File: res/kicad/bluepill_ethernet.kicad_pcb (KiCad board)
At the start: 2 copper layers, 50.4 x 48 mm, 23 parts, among them J1 HEADER-1x20, J2 Conn_01x03, J3 Conn_02x05_Odd_Even, SW1 SW_Push, U1 BluePill_STM32F103C, U2 93C46, U3 WIZ850io

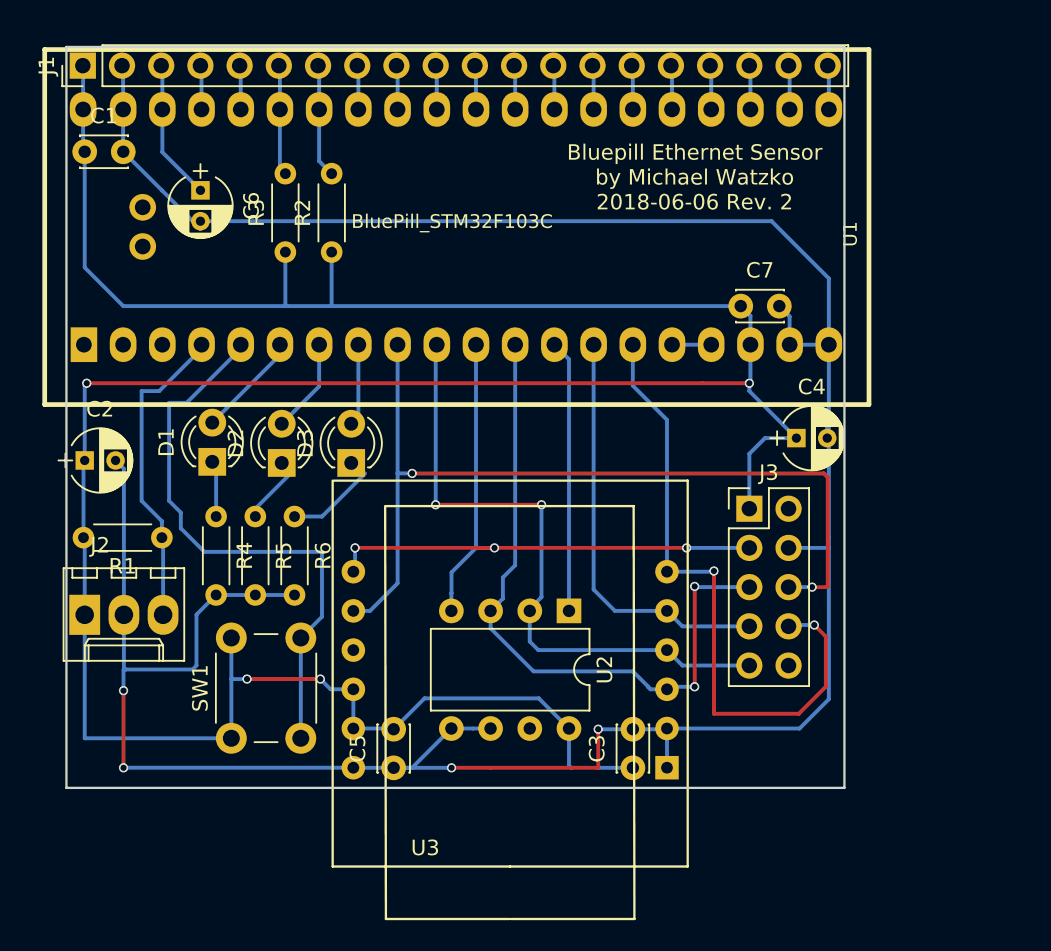
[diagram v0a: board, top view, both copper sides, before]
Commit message: board revision 3 alpha 1
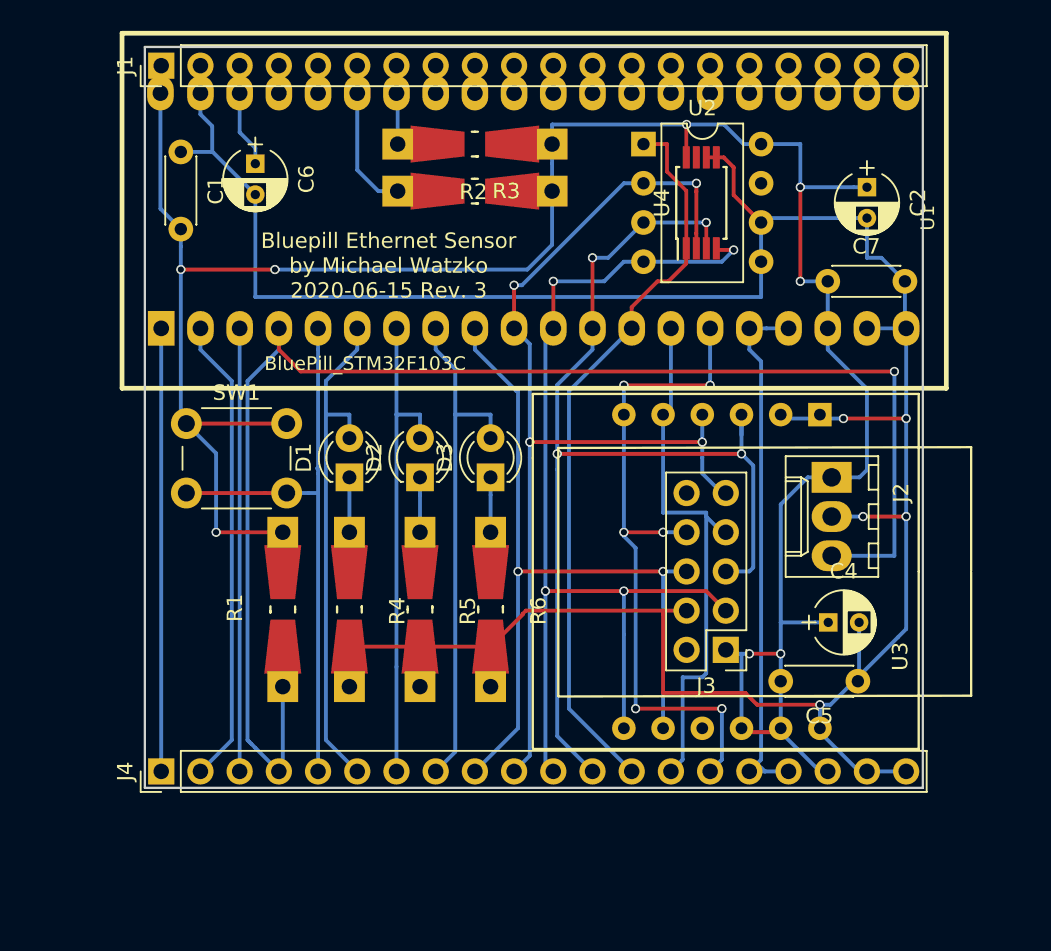
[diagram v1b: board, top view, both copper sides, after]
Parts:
- removed C3: C, Capacitors_THT:C_Disc_D3.0mm_W2.0mm_P2.50mm
- added J4: HEADER-1x20, Pin_Headers:Pin_Header_Straight_1x20_Pitch2.54mm, F.Cu at (43.9, 78.2)
- added U4: 93C46, Housings_SSOP:TSSOP-8_4.4x3mm_Pitch0.65mm, F.Cu at (78.9, 41.4)
- C1, C5, C7: footprint Capacitors_THT:C_Disc_D3.0mm_W2.0mm_P2.50mm -> Capacitors_THT:C_Disc_D4.3mm_W1.9mm_P5.00mm
- R1, R2, R3, R4, R5, R6: footprint Resistors_THT:R_Axial_DIN0204_L3.6mm_D1.6mm_P5.08mm_Horizontal -> Resistors_Universal:Resistor_SMD+THTuniversal_0805to1206_RM10_HandSoldering
- moved C2 53.7 mm to (89.7, 40.4), turned to 270 degrees
- moved J2 49.2 mm to (87.4, 59.2), turned to 270 degrees
- moved U2 30.6 mm to (75.2, 37.6), turned to 0 degrees
- moved C5 30.6 mm to (89.1, 72.4), turned to 180 degrees
- moved U3 23.8 mm to (86.6, 65.3), turned to 270 degrees
- moved SW1 20.6 mm to (45.6, 55.7), turned to 0 degrees
- moved R6 14.1 mm to (65.3, 67.7)
- moved R3 12.9 mm to (64.3, 40.6), turned to 180 degrees
- moved R5 12.2 mm to (60.7, 67.7)
- moved C4 12.1 mm to (87.2, 68.6)
- moved R2 11.6 mm to (64.3, 37.6), turned to 180 degrees
- moved R4 10.5 mm to (56.1, 67.7)
- moved J3 9.27 mm to (80.5, 70.4), turned to 180 degrees
- moved R1 9.11 mm to (51.8, 67.7), turned to 90 degrees
- moved D3 9.08 mm to (65.3, 59.2)
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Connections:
- C1 pad 1: VCC -> GND
- C1 pad 2: GND -> VCC
- D1 pad 2: Net-(D1-Pad2) -> (no net)
- D2 pad 2: Net-(D2-Pad2) -> (no net)
- D3 pad 2: Net-(D3-Pad2) -> (no net)
- U1 pad 1: (no net) -> Net-(BT1-Pad1)
- U1 pad 2: (no net) -> Net-(J4-Pad2)
- U1 pad 3: (no net) -> Net-(J4-Pad3)
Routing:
- net Net-(J2-Pad3): track 21.2 -> 96.4 mm, vias 0 -> 1
- net Net-(J4-Pad16): track 2.54 -> 34.8 mm
- net Net-(J4-Pad2): track 0.00 -> 30.4 mm
- net Net-(J4-Pad13): track 17.6 -> 47.9 mm
- net Net-(BT1-Pad1): track 0.00 -> 28.8 mm
- net Net-(J4-Pad3): track 0.00 -> 28.7 mm
- net Net-(D3-Pad2): track 5.31 -> 33.6 mm
- net Net-(J3-Pad9): track 41.2 -> 68.0 mm, vias 2 -> 4
- net Net-(D1-Pad2): track 6.87 -> 33.4 mm
- net VCC: track 195.8 -> 169.5 mm, vias 4 -> 8
- net Net-(J3-Pad5): track 44.0 -> 70.3 mm, vias 2 -> 4
- net Net-(D2-Pad2): track 6.13 -> 31.8 mm
- net Net-(J3-Pad3): track 46.2 -> 67.2 mm, vias 3 -> 4
- net Net-(J3-Pad7): track 26.9 -> 35.4 mm
- net GND: track 185.5 -> 178.9 mm, vias 4 -> 5
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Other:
- board text added: "Bluepill Ethernet Sensor by Michael Watzko 2020-06-15 Rev. 3"
- board text removed: "Bluepill Ethernet Sensor by Michael Watzko 2018-06-06 Rev. 2"

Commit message: Board Rev 3.0
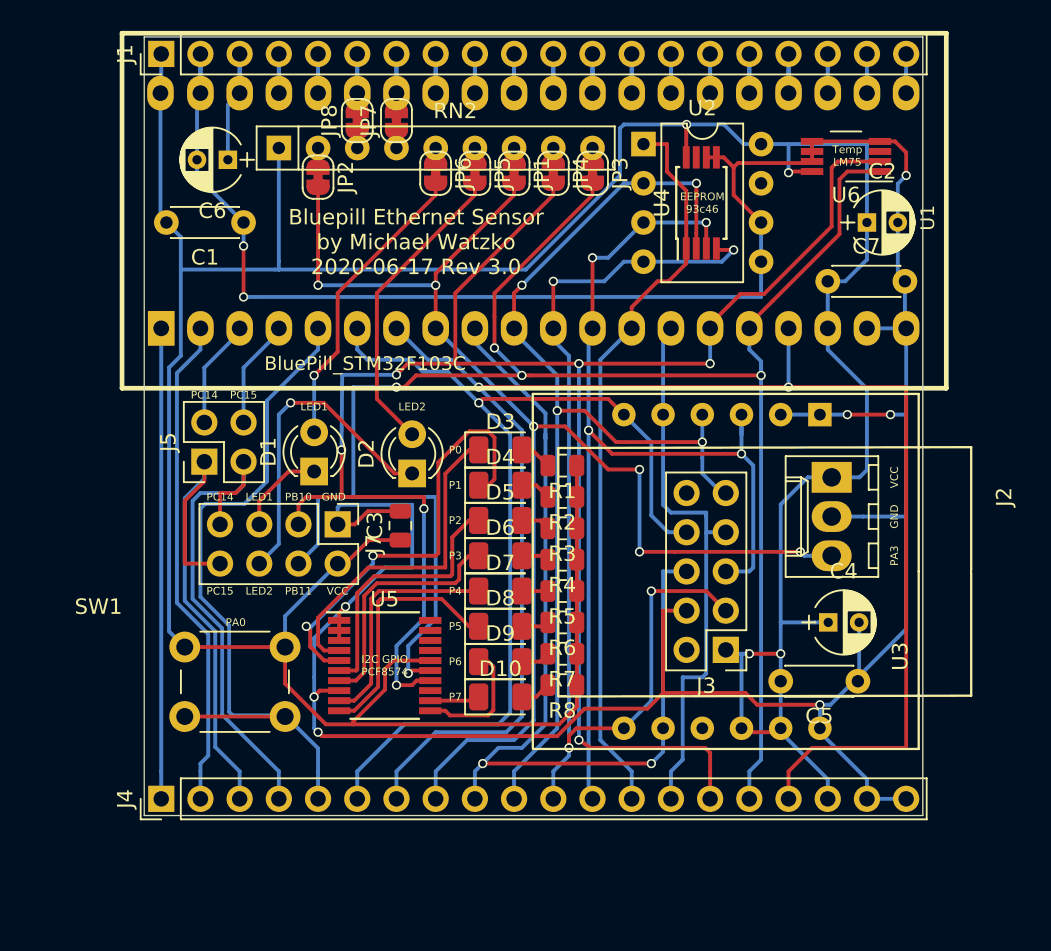
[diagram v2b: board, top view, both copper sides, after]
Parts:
- added C3: C, Capacitor_SMD:C_0805_2012Metric, F.Cu at (59.4, 62.3)
- added D10: LED, LED_SMD:LED_1206_3216Metric, F.Cu at (65.9, 73.4)
- added D4: LED, LED_SMD:LED_1206_3216Metric, F.Cu at (65.9, 59.7)
- added D5: LED, LED_SMD:LED_1206_3216Metric, F.Cu at (65.9, 62.0)
- added D6: LED, LED_SMD:LED_1206_3216Metric, F.Cu at (65.9, 64.3)
- added D7: LED, LED_SMD:LED_1206_3216Metric, F.Cu at (65.9, 66.5)
- added D8: LED, LED_SMD:LED_1206_3216Metric, F.Cu at (65.9, 68.8)
- added D9: LED, LED_SMD:LED_1206_3216Metric, F.Cu at (65.9, 71.1)
- added J5: Conn_02x02_Odd_Even, Connector_PinHeader_2.54mm:PinHeader_2x02_P2.54mm_Vertical, F.Cu at (46.7, 58.2)
- added J7: Conn_02x04_Odd_Even, Connector_PinHeader_2.54mm:PinHeader_2x04_P2.54mm_Vertical, F.Cu at (55.4, 62.2)
- added JP1: SolderJumper_2_Bridged, Jumper:SolderJumper-2_P1.3mm_Bridged_RoundedPad1.0x1.5mm, F.Cu at (66.8, 39.5)
- added JP2: SolderJumper_2_Bridged, Jumper:SolderJumper-2_P1.3mm_Bridged_RoundedPad1.0x1.5mm, F.Cu at (54.1, 39.7)
- added JP3: SolderJumper_2_Bridged, Jumper:SolderJumper-2_P1.3mm_Bridged_RoundedPad1.0x1.5mm, F.Cu at (71.9, 39.5)
- added JP4: SolderJumper_2_Bridged, Jumper:SolderJumper-2_P1.3mm_Bridged_RoundedPad1.0x1.5mm, F.Cu at (69.3, 39.5)
- added JP5: SolderJumper_2_Bridged, Jumper:SolderJumper-2_P1.3mm_Bridged_RoundedPad1.0x1.5mm, F.Cu at (64.3, 39.5)
- added JP6: SolderJumper_2_Bridged, Jumper:SolderJumper-2_P1.3mm_Bridged_RoundedPad1.0x1.5mm, F.Cu at (61.7, 39.5)
- added JP7: SolderJumper_2_Bridged, Jumper:SolderJumper-2_P1.3mm_Bridged_RoundedPad1.0x1.5mm, F.Cu at (59.2, 36.1)
- added JP8: SolderJumper_2_Bridged, Jumper:SolderJumper-2_P1.3mm_Bridged_RoundedPad1.0x1.5mm, F.Cu at (56.6, 36.1)
- added R7: R, Resistor_SMD:R_0805_2012Metric, F.Cu at (69.9, 70.6)
- added R8: R, Resistor_SMD:R_0805_2012Metric, F.Cu at (69.9, 72.6)
- added RN2: 4,7k, Resistor_THT:R_Array_SIP9, F.Cu at (51.6, 37.8)
- added U5: PCF8574A, Package_SO:TSSOP-20_4.4x6.5mm_P0.65mm, F.Cu at (58.4, 71.4)
- added U6: LM75B, Package_SO:VSSOP-8_3.0x3.0mm_P0.65mm, F.Cu at (88.3, 38.4)
- D1, D2: footprint LEDs:LED_D3.0mm -> LED_THT:LED_D3.0mm
- D3: footprint LEDs:LED_D3.0mm -> LED_SMD:LED_1206_3216Metric
- R1, R2, R3, R4, R5, R6: footprint Resistors_Universal:Resistor_SMD+THTuniversal_0805to1206_RM10_HandSoldering -> Resistor_SMD:R_0805_2012Metric
- moved R2 23.6 mm to (69.9, 60.5)
- moved R3 22.6 mm to (69.9, 62.5)
- moved R1 20.4 mm to (69.9, 58.4), turned to 180 degrees
- moved SW1 14.5 mm to (45.5, 70.2)
- moved R4 14.2 mm to (69.9, 64.5), turned to 180 degrees
- moved R5 9.30 mm to (69.9, 66.5), turned to 180 degrees
- moved C1 6.12 mm to (49.3, 42.7), turned to 180 degrees
- moved R6 4.73 mm to (69.9, 68.6), turned to 180 degrees
- moved D1 2.32 mm to (53.8, 58.8)
- moved C2 2.29 mm to (89.7, 42.7), turned to 0 degrees
- moved D3 1.89 mm to (65.9, 57.4), turned to 0 degrees
- moved C6 1.80 mm to (48.3, 38.6), turned to 180 degrees
- moved J4 1.78 mm to (43.9, 80.0)
- moved J1 0.76 mm to (43.9, 31.8)
- moved D2 0.57 mm to (60.2, 58.9)
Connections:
- D1 pad 2: (no net) -> dled1
- D2 pad 2: (no net) -> dled2
- D3 pad 2: (no net) -> Net-(D3-Pad2)
- J4 pad 15: Net-(J3-Pad8) -> i2c1c
- J4 pad 16: Net-(J4-Pad16) -> i2c1d
- J4 pad 17: Net-(J4-Pad16) -> Net-(J4-Pad17)
- J4 pad 4: Net-(J2-Pad3) -> Net-(J4-Pad4)
- J4 pad 6: Net-(D1-Pad2) -> Net-(J3-Pad8)
- J4 pad 7: Net-(D2-Pad2) -> Net-(J4-Pad17)
- J4 pad 8: Net-(D3-Pad2) -> Net-(J2-Pad3)
- R1 pad 1: Net-(J2-Pad3) -> VCC
- R1 pad 2: VCC -> Net-(D3-Pad2)
- R2 pad 2: Net-(J1-Pad7) -> Net-(D4-Pad2)
- R3 pad 2: Net-(J1-Pad6) -> Net-(D5-Pad2)
- R4 pad 1: Net-(D1-Pad1) -> VCC
- R4 pad 2: GND -> Net-(D6-Pad2)
- R5 pad 1: Net-(D2-Pad1) -> VCC
- R5 pad 2: GND -> Net-(D7-Pad2)
- R6 pad 1: Net-(D3-Pad1) -> VCC
- R6 pad 2: GND -> Net-(D8-Pad2)
- U1 pad 15: Net-(J3-Pad8) -> i2c1c
- U1 pad 16: Net-(J4-Pad16) -> i2c1d
- U1 pad 17: Net-(J4-Pad16) -> Net-(J4-Pad17)
- U1 pad 3: Net-(J4-Pad3) -> Net-(J5-Pad2)
- U1 pad 4: Net-(J2-Pad3) -> Net-(J5-Pad4)
- U1 pad 6: Net-(D1-Pad2) -> Net-(J3-Pad8)
- U1 pad 7: Net-(D2-Pad2) -> Net-(J4-Pad17)
- U1 pad 8: Net-(D3-Pad2) -> Net-(J2-Pad3)
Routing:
- net i2c1c: track 0.00 -> 127.5 mm, vias 0 -> 7
- net i2c1d: track 0.00 -> 122.7 mm, vias 0 -> 5
- net Net-(J4-Pad17): track 0.00 -> 105.7 mm, vias 0 -> 2
- net VCC: track 169.5 -> 233.3 mm, vias 8 -> 4
- net GND: track 178.9 -> 219.5 mm, vias 5 -> 9
- net Net-(J4-Pad16): track 34.8 -> 0.00 mm
- net Net-(D1-Pad2): track 33.4 -> 0.00 mm
- net Net-(J4-Pad4): track 0.00 -> 32.2 mm
- net Net-(D2-Pad2): track 31.8 -> 0.00 mm
- net Net-(D3-Pad2): track 33.6 -> 2.10 mm
- net Net-(D4-Pad1): track 0.00 -> 29.2 mm, vias 0 -> 2
- net Net-(J3-Pad8): track 44.3 -> 64.8 mm, vias 6 -> 1
- net dled2: track 0.00 -> 19.8 mm
- net dled1: track 0.00 -> 19.4 mm, vias 0 -> 1
- net Net-(D5-Pad1): track 0.00 -> 17.4 mm
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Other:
- board size 50.4 x 48 mm -> 50.4 x 50.4 mm
- board text added: "Bluepill Ethernet Sensor by Michael Watzko 2020-06-17 Rev 3.0"
- board text added: "EEPROM 93c46"
- board text added: "GND"
- board text added: "I2C GPIO PCF8574"
- board text added: "LED1"
- board text added: "LED2"
- board text added: "P0"
- board text added: "P1"
- board text added: "P2"
- board text added: "P3"
- board text added: "P4"
- board text added: "P5"
- board text added: "P6"
- board text added: "P7"
- board text added: "PA0"
- board text added: "PA3"
- board text added: "PB10"
- board text added: "PB11"
- board text added: "PC14"
- board text added: "PC15"
- board text added: "Temp LM75"
- board text added: "VCC"
- board text removed: "Bluepill Ethernet Sensor by Michael Watzko 2020-06-15 Rev. 3"
